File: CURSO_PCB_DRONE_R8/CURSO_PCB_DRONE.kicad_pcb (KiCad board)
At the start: 4 copper layers, 102 x 49 mm, 163 parts, among them J1 USB_B_Micro, J10 CONN_MOT_1, J11 CONN_MOT_3, J12 LIDAR, J13 CONN_STM32_I2C, J14 CONN_MOT_2, J15 CONN_MOT_4, J16 Conn_Coaxial, J17 XT-60, J2 SWD, J3 USB_B_Micro, J4 ICSP, J5 OLED, J6 CONN_STM32_USART, J7 jumper, J8 CONN_MANDO, J9 CONN_STM32_SPI, SW1 RST, SW2 RST, SW3 RST, SW4 SW_Push_SPDT, U1 CH340G, U10 MPU-6050, U11 LM7805_TO220, U12 AMS1117-3.3, U2 ATMEGA328P-AU, U3 LM358DR, U4 STM32F103R8T6, U5 nRF24L01P, U6 74HC245, U7 MICROSD_C164170, U8 SRV05-4, U9 74AHC1G125, Y1 16Mhz, Y2 12Mhz, Y3 8Mhz, Y4 32.768kHz, Y5 16Mhz

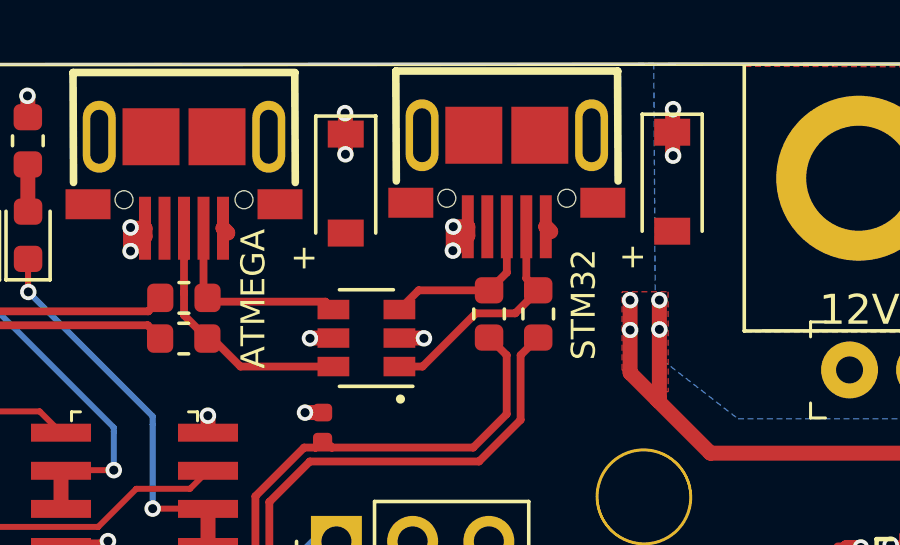
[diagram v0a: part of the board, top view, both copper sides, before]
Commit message: Add files via upload
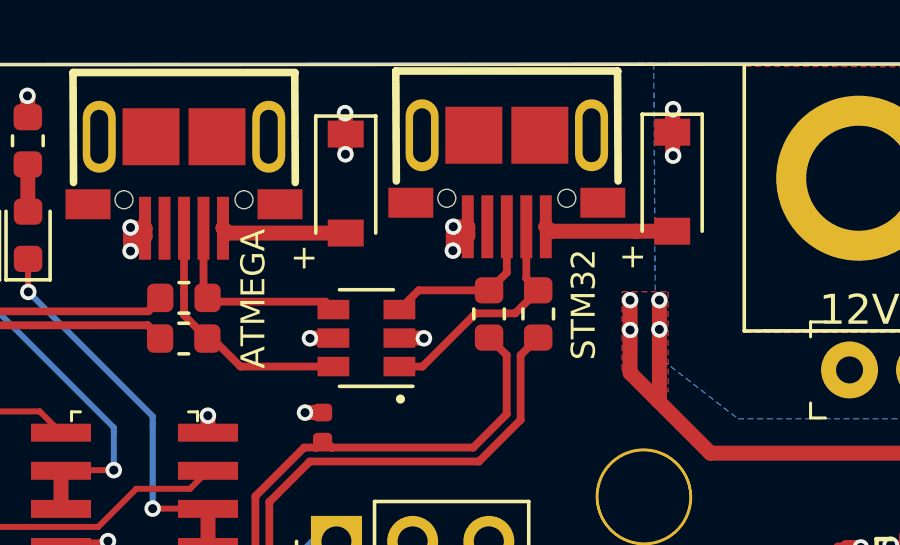
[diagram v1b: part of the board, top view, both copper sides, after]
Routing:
- net Net-(D9-Pad2): track 0.45 -> 4.51 mm
- net Net-(D1-Pad2): track 0.44 -> 4.37 mm
